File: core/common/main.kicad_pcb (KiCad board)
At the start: 2 copper layers, 42.7 x 25.7 mm, 6 parts, among them P1 CONN_01X05, P2 CONN_01X03, P3 CONN_01X02, P4 CONN_01X02, U1 NDSL_DPad, U2 NDSL_SS

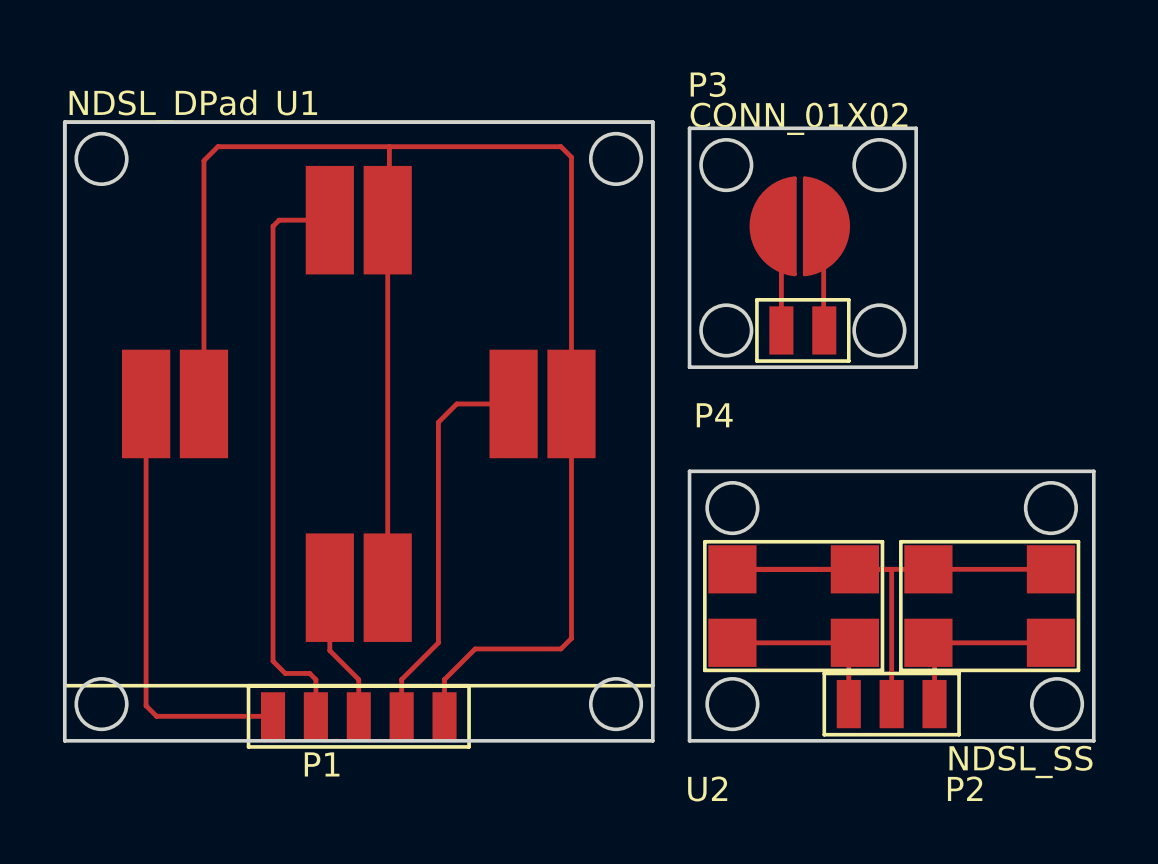
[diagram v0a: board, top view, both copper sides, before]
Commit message: updated core/common
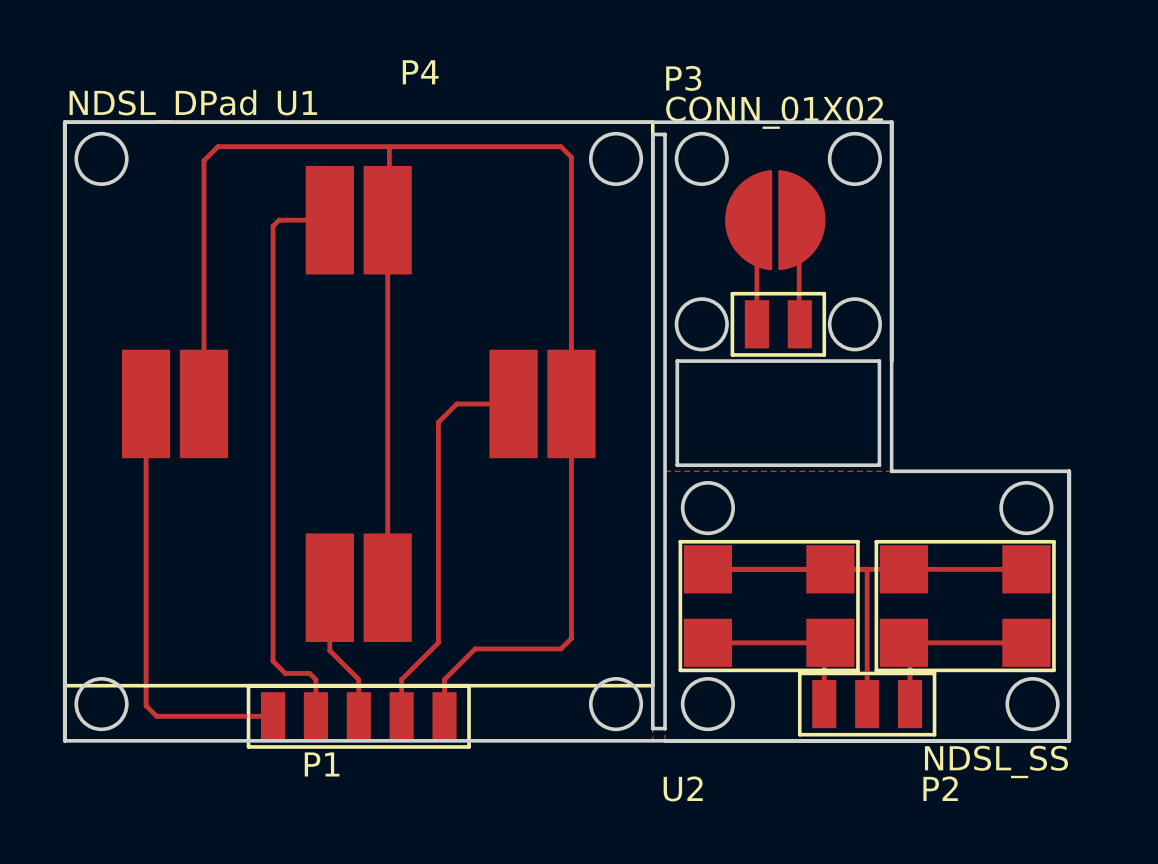
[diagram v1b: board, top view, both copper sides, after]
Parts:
- moved P3 1.05 mm to (143.0, 110.5)
- moved P4 1.05 mm to (143.0, 115.8)
- moved P2 1.02 mm to (146.8, 131.6)
- moved U2 1.02 mm to (146.8, 126.5)
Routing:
- added copper zone on F.Cu, net DC
- added copper zone on F.Cu, net SC
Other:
- board size 42.7 x 25.7 mm -> 41.7 x 25.7 mm
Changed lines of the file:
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@@
     (links 18)
     (no_connects 0)
-    (area 113.076667 103.927 156.600096 135.187)
+    (area 113.076667 103.419 155.584096 135.187)
     (thickness 1.6)
-    (drawings 24)
+    (drawings 30)
     (tracks 47)
     (zones 0)
@@
   )
   (module steward:MyFT_SIM3 (layer F.Cu)
-    (at 147.828 131.572)
+    (at 146.812 131.572)
     (attr smd)
     (fp_text reference P2 (at 3.048 2.54) (layer F.SilkS)
@@
   )
   (module steward:MyFT_SIM2 (layer F.Cu)
-    (at 144.018 116.078)
+    (at 143.002 115.824)
     (attr smd)
-    (fp_text reference P4 (at -3.556 2.54) (layer F.SilkS)
-      (effects (font (size 1 1) (thickness 0.15)))
-    )
-    (fp_text value CONN_01X02 (at 0.254 1.27) (layer F.Fab)
+    (fp_text reference P4 (at -14.732 -11.43) (layer F.SilkS)
+      (effects (font (size 1 1) (thickness 0.15)))
+    )
+    (fp_text value CONN_01X02 (at -10.922 -10.16) (layer F.Fab)
       (effects (font (size 1 1) (thickness 0.15)))
     )
@@
   )
   (module steward:MyFT_Pad_Circle (layer F.Cu)
-    (at 144.018 110.744)
+    (at 143.002 110.49)
     (descr GamePad)
     (tags GamePad)
@@
   )
   (module steward:MyFT_NDSL_SS (layer F.Cu)
-    (at 147.828 126.492 180)
+    (at 146.812 126.492 180)
     (descr "NDSL SS")
     (tags "NDSL SS")
@@
     )
   )
-  (gr_line (start 139.446 116.586) (end 148.844 116.586) (angle 90) (layer Edge.Cuts) (width 0.15))
-  (gr_line (start 148.844 106.68) (end 139.446 106.68) (angle 90) (layer Edge.Cuts) (width 0.15))
-  (gr_line (start 139.446 116.586) (end 139.446 106.68) (angle 90) (layer Edge.Cuts) (width 0.15))
-  (gr_line (start 148.844 106.68) (end 148.844 116.586) (angle 90) (layer Edge.Cuts) (width 0.15))
-  (gr_circle (center 147.32 108.204) (end 148.336 108.458) (layer Edge.Cuts) (width 0.15))
-  (gr_circle (center 147.32 115.062) (end 148.336 115.316) (layer Edge.Cuts) (width 0.15))
-  (gr_line (start 139.446 132.08) (end 139.446 120.904) (angle 90) (layer Edge.Cuts) (width 0.15))
-  (gr_line (start 156.21 120.904) (end 156.21 132.08) (angle 90) (layer Edge.Cuts) (width 0.15))
-  (gr_line (start 156.21 132.08) (end 139.446 132.08) (angle 90) (layer Edge.Cuts) (width 0.15))
-  (gr_line (start 139.446 120.904) (end 156.21 120.904) (angle 90) (layer Edge.Cuts) (width 0.15))
-  (gr_circle (center 140.97 115.062) (end 141.986 115.316) (layer Edge.Cuts) (width 0.15))
-  (gr_circle (center 140.97 108.204) (end 141.986 108.458) (layer Edge.Cuts) (width 0.15))
-  (gr_circle (center 141.224 122.428) (end 142.24 122.682) (layer Edge.Cuts) (width 0.15))
-  (gr_circle (center 154.432 122.428) (end 155.448 122.682) (layer Edge.Cuts) (width 0.15))
-  (gr_circle (center 154.686 130.556) (end 155.702 130.81) (layer Edge.Cuts) (width 0.15))
-  (gr_circle (center 141.224 130.556) (end 142.24 130.81) (layer Edge.Cuts) (width 0.15))
+  (gr_line (start 138.938 120.65) (end 147.32 120.65) (angle 90) (layer Edge.Cuts) (width 0.15))
+  (gr_line (start 138.938 116.332) (end 147.32 116.332) (angle 90) (layer Edge.Cuts) (width 0.15))
+  (gr_line (start 147.32 116.332) (end 147.32 120.65) (angle 90) (layer Edge.Cuts) (width 0.15))
+  (gr_line (start 138.938 116.332) (end 138.938 120.65) (angle 90) (layer Edge.Cuts) (width 0.15))
+  (gr_line (start 138.43 106.934) (end 138.43 131.572) (angle 90) (layer Edge.Cuts) (width 0.15))
+  (gr_line (start 137.922 131.572) (end 137.922 106.934) (angle 90) (layer Edge.Cuts) (width 0.15))
+  (gr_line (start 138.43 131.572) (end 137.922 131.572) (angle 90) (layer Edge.Cuts) (width 0.15))
+  (gr_line (start 137.922 106.934) (end 138.43 106.934) (angle 90) (layer Edge.Cuts) (width 0.15))
+  (gr_line (start 113.538 132.08) (end 113.538 106.426) (angle 90) (layer Edge.Cuts) (width 0.15))
+  (gr_line (start 155.194 132.08) (end 113.538 132.08) (angle 90) (layer Edge.Cuts) (width 0.15))
+  (gr_line (start 155.194 120.904) (end 155.194 132.08) (angle 90) (layer Edge.Cuts) (width 0.15))
+  (gr_line (start 147.828 120.904) (end 155.194 120.904) (angle 90) (layer Edge.Cuts) (width 0.15))
+  (gr_line (start 147.828 106.426) (end 147.828 120.904) (angle 90) (layer Edge.Cuts) (width 0.15))
+  (gr_line (start 113.538 106.426) (end 147.828 106.426) (angle 90) (layer Edge.Cuts) (width 0.15))
+  (gr_line (start 147.828 106.426) (end 147.828 116.332) (angle 90) (layer Edge.Cuts) (width 0.15))
+  (gr_circle (center 146.304 107.95) (end 147.32 108.204) (layer Edge.Cuts) (width 0.15))
+  (gr_circle (center 146.304 114.808) (end 147.32 115.062) (layer Edge.Cuts) (width 0.15))
+  (gr_line (start 155.194 120.904) (end 155.194 132.08) (angle 90) (layer Edge.Cuts) (width 0.15))
+  (gr_line (start 155.194 132.08) (end 138.43 132.08) (angle 90) (layer Edge.Cuts) (width 0.15))
+  (gr_circle (center 139.954 114.808) (end 140.97 115.062) (layer Edge.Cuts) (width 0.15))
+  (gr_circle (center 139.954 107.95) (end 140.97 108.204) (layer Edge.Cuts) (width 0.15))
+  (gr_circle (center 140.208 122.428) (end 141.224 122.682) (layer Edge.Cuts) (width 0.15))
+  (gr_circle (center 153.416 122.428) (end 154.432 122.682) (layer Edge.Cuts) (width 0.15))
+  (gr_circle (center 153.67 130.556) (end 154.686 130.81) (layer Edge.Cuts) (width 0.15))
+  (gr_circle (center 140.208 130.556) (end 141.224 130.81) (layer Edge.Cuts) (width 0.15))
   (gr_circle (center 136.398 130.556) (end 137.414 130.81) (layer Edge.Cuts) (width 0.15))
   (gr_circle (center 115.062 130.556) (end 116.078 130.81) (layer Edge.Cuts) (width 0.15))
@@
   (gr_circle (center 115.062 107.95) (end 116.078 108.204) (layer Edge.Cuts) (width 0.15))
   (gr_line (start 113.538 132.08) (end 113.538 106.426) (angle 90) (layer Edge.Cuts) (width 0.15))
-  (gr_line (start 137.922 132.08) (end 113.538 132.08) (angle 90) (layer Edge.Cuts) (width 0.15))
-  (gr_line (start 137.922 106.426) (end 137.922 132.08) (angle 90) (layer Edge.Cuts) (width 0.15))
-  (gr_line (start 113.538 106.426) (end 137.922 106.426) (angle 90) (layer Edge.Cuts) (width 0.15))
   (segment (start 116.91 118.11) (end 116.91 130.626) (width 0.2) (layer F.Cu) (net 1))
   (segment (start 117.348 131.064) (end 122.174 131.064) (width 0.2) (layer F.Cu) (net 1))
@@
   (segment (start 119.31 108.02) (end 119.888 107.442) (width 0.2) (layer F.Cu) (net 5))
   (segment (start 126.93 125.73) (end 126.93 110.49) (width 0.2) (layer F.Cu) (net 5))
-  (segment (start 147.828 130.556) (end 147.828 124.968) (width 0.2) (layer F.Cu) (net 6))
-  (segment (start 147.828 124.968) (end 141.224 124.968) (width 0.2) (layer F.Cu) (net 6))
-  (segment (start 141.224 124.968) (end 146.304 124.968) (width 0.2) (layer F.Cu) (net 6))
-  (segment (start 146.304 124.968) (end 149.352 124.968) (width 0.2) (layer F.Cu) (net 6))
-  (segment (start 149.352 124.968) (end 154.432 124.968) (width 0.2) (layer F.Cu) (net 6))
-  (segment (start 141.224 128.016) (end 146.304 128.016) (width 0.2) (layer F.Cu) (net 7))
-  (segment (start 146.304 128.016) (end 146.05 128.27) (width 0.2) (layer F.Cu) (net 7))
-  (segment (start 146.05 128.27) (end 146.05 130.556) (width 0.2) (layer F.Cu) (net 7))
-  (segment (start 149.606 130.556) (end 149.606 128.27) (width 0.2) (layer F.Cu) (net 8))
-  (segment (start 149.606 128.27) (end 149.86 128.016) (width 0.2) (layer F.Cu) (net 8))
-  (segment (start 149.86 128.016) (end 154.432 128.016) (width 0.2) (layer F.Cu) (net 8))
-  (segment (start 143.256 115.062) (end 143.256 110.9726) (width 0.2) (layer F.Cu) (net 9))
-  (segment (start 143.256 110.9726) (end 143.0274 110.744) (width 0.2) (layer F.Cu) (net 9))
-  (segment (start 145.0086 110.744) (end 145.0086 115.0366) (width 0.2) (layer F.Cu) (net 10))
-  (segment (start 145.0086 115.0366) (end 145.034 115.062) (width 0.2) (layer F.Cu) (net 10))
+  (segment (start 146.812 130.556) (end 146.812 124.968) (width 0.2) (layer F.Cu) (net 6))
+  (segment (start 146.812 124.968) (end 140.208 124.968) (width 0.2) (layer F.Cu) (net 6))
+  (segment (start 140.208 124.968) (end 145.288 124.968) (width 0.2) (layer F.Cu) (net 6))
+  (segment (start 145.288 124.968) (end 148.336 124.968) (width 0.2) (layer F.Cu) (net 6))
+  (segment (start 148.336 124.968) (end 153.416 124.968) (width 0.2) (layer F.Cu) (net 6))
+  (segment (start 140.208 128.016) (end 145.288 128.016) (width 0.2) (layer F.Cu) (net 7))
+  (segment (start 145.288 128.016) (end 145.034 128.27) (width 0.2) (layer F.Cu) (net 7))
+  (segment (start 145.034 128.27) (end 145.034 130.556) (width 0.2) (layer F.Cu) (net 7))
+  (segment (start 148.59 130.556) (end 148.59 128.27) (width 0.2) (layer F.Cu) (net 8))
+  (segment (start 148.59 128.27) (end 148.844 128.016) (width 0.2) (layer F.Cu) (net 8))
+  (segment (start 148.844 128.016) (end 153.416 128.016) (width 0.2) (layer F.Cu) (net 8))
+  (segment (start 142.24 114.808) (end 142.24 110.7186) (width 0.2) (layer F.Cu) (net 9))
+  (segment (start 142.24 110.7186) (end 142.0114 110.49) (width 0.2) (layer F.Cu) (net 9))
+  (segment (start 143.9926 110.49) (end 143.9926 114.7826) (width 0.2) (layer F.Cu) (net 10))
+  (segment (start 143.9926 114.7826) (end 144.018 114.808) (width 0.2) (layer F.Cu) (net 10))
+  (zone (net 6) (net_name SC) (layer F.Cu) (hatch edge 0.508)
+    (connect_pads (clearance 0.508))
+    (min_thickness 0.254)
+    (fill yes (arc_segments 16) (thermal_gap 0.508) (thermal_bridge_width 0.508))
+    (polygon
+      (pts
+        (xy 155.194 132.08) (xy 138.43 132.08) (xy 138.43 120.904) (xy 155.194 120.904)
+      )
+    )
+  )
+  (zone (net 5) (net_name DC) (layer F.Cu) (hatch edge 0.508)
+    (connect_pads (clearance 0.508))
+    (min_thickness 0.254)
+    (fill yes (arc_segments 16) (thermal_gap 0.508) (thermal_bridge_width 0.508))
+    (polygon
+      (pts
+        (xy 137.922 132.08) (xy 113.538 132.08) (xy 113.538 106.426) (xy 137.922 106.426)
+      )
+    )
+  )
 )

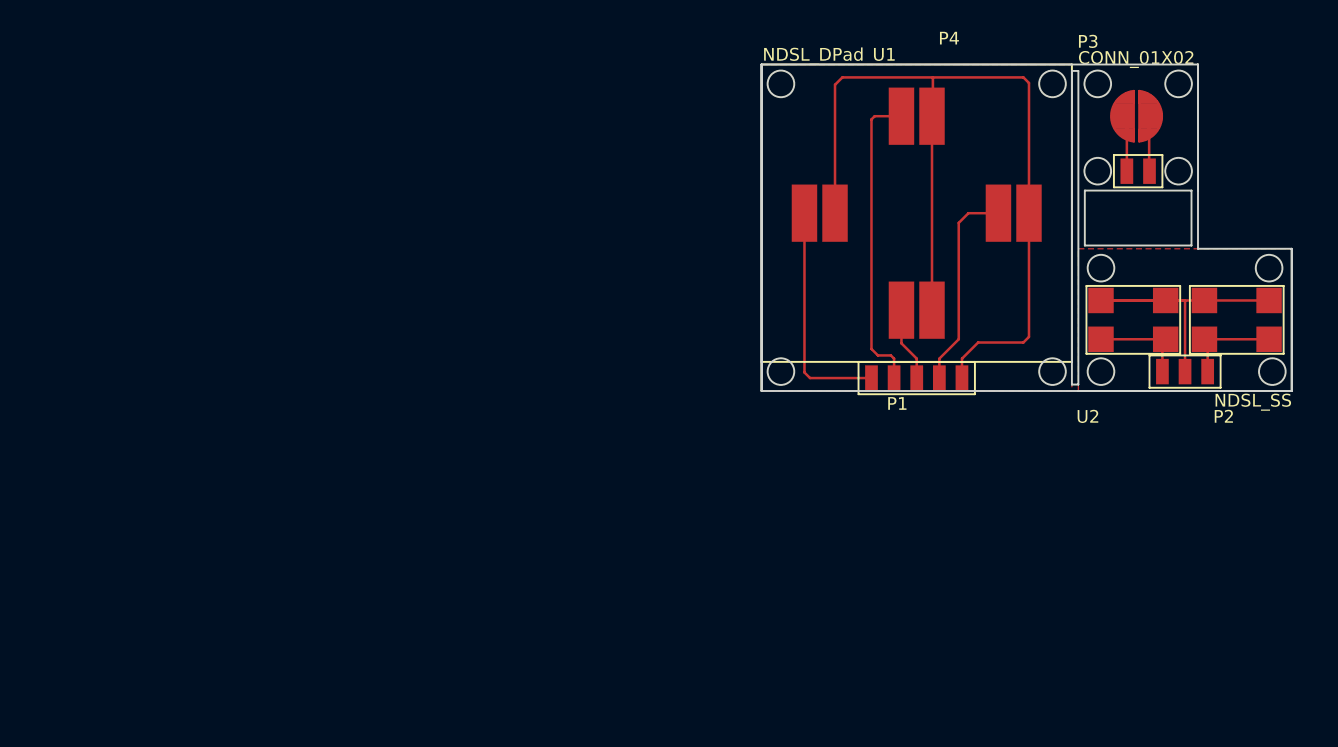
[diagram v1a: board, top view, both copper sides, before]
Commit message: updated for ndsl_dpad, ndsl_ss, ndsl_lr, n900_keyboard
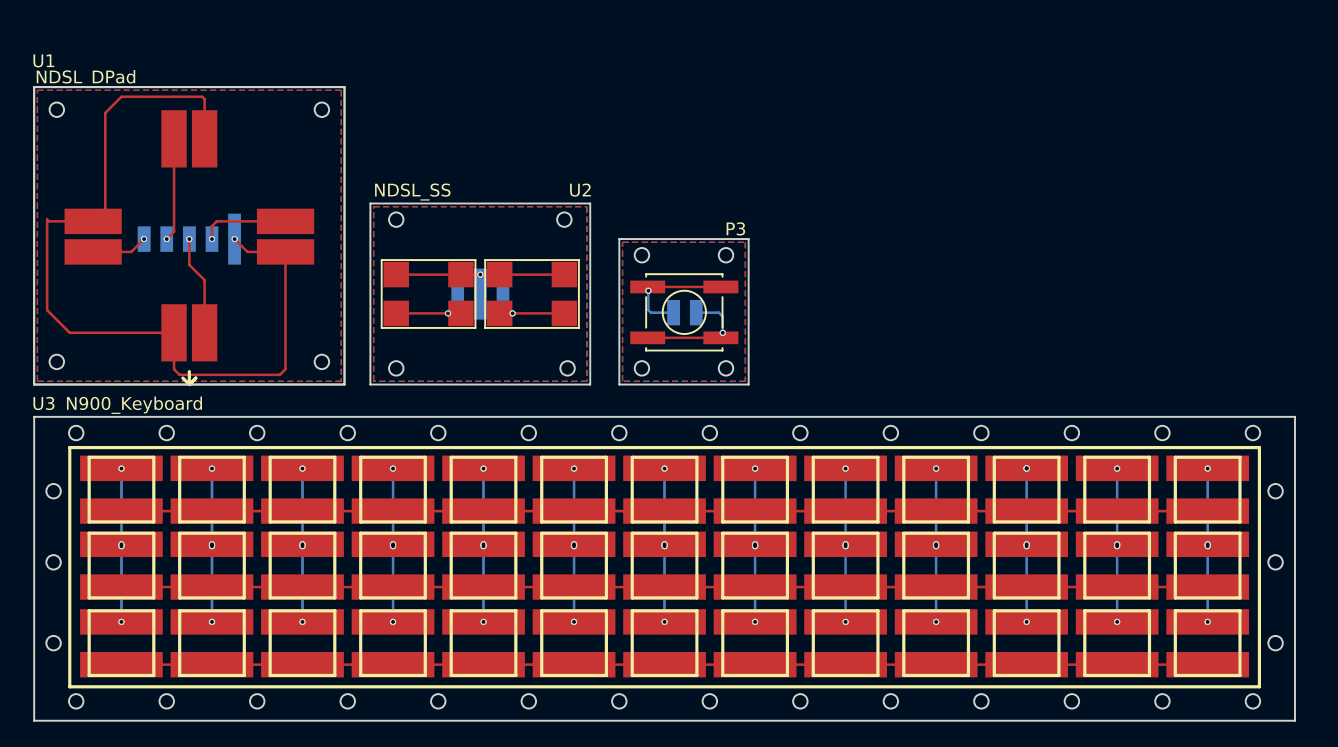
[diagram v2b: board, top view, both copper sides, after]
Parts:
- added U3: N900_Keyboard, steward:MyFT_N900_Keyboard, F.Cu at (102.6, 145.5)
- P1, P2, P4: moved to B.Cu
- P3: footprint steward:MyFT_Pad_Circle -> Buttons_Switches_SMD:SW_SPST_EVPBF
- moved P1 58.6 mm to (68.6, 119.1)
- moved U1 57.9 mm to (68.6, 119.9)
- moved P2 56.0 mm to (91.4, 123.4)
- moved U2 55.4 mm to (91.4, 124.5)
- moved P3 38.7 mm to (107.5, 125.9)
- moved P4 36.8 mm to (107.4, 124.9)
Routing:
- net Net-(U3-Pad16): track 0.00 -> 85.3 mm
- net Net-(U3-Pad14): track 0.00 -> 85.3 mm
- net Net-(U3-Pad15): track 0.00 -> 85.3 mm
- net DU: track 24.1 -> 8.11 mm, vias 0 -> 1
- net DL: track 18.0 -> 4.42 mm, vias 0 -> 1
- net Net-(U3-Pad11): track 0.00 -> 12.1 mm, vias 0 -> 5
- net Net-(U3-Pad9): track 0.00 -> 12.1 mm, vias 0 -> 4
- net Net-(U3-Pad8): track 0.00 -> 12.1 mm, vias 0 -> 4
- net Net-(U3-Pad7): track 0.00 -> 12.1 mm, vias 0 -> 4
- net Net-(U3-Pad6): track 0.00 -> 12.1 mm, vias 0 -> 4
- net Net-(U3-Pad5): track 0.00 -> 12.1 mm, vias 0 -> 4
- net Net-(U3-Pad4): track 0.00 -> 12.1 mm, vias 0 -> 4
- net Net-(U3-Pad3): track 0.00 -> 12.1 mm, vias 0 -> 4
- net Net-(U3-Pad2): track 0.00 -> 12.1 mm, vias 0 -> 4
- net Net-(U3-Pad13): track 0.00 -> 12.1 mm, vias 0 -> 4
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- added copper zone on F.Cu, net B1
- added copper zone on B.Cu, net B2
- added copper zone on B.Cu, net DC
- added copper zone on B.Cu, net SC
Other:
- board size 41.7 x 25.7 mm -> 99.1 x 49.8 mm
